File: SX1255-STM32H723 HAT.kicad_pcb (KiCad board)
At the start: 2 copper layers, 77 x 44.2 mm, 36 parts, among them IC1 SX1255, J1 TX_ANT, J2 RX_ANT, J3 STM-L, J4 STM-R, U1 MCP1703Ax-330xxMB, X1 TA0692A, Y1 32MHz

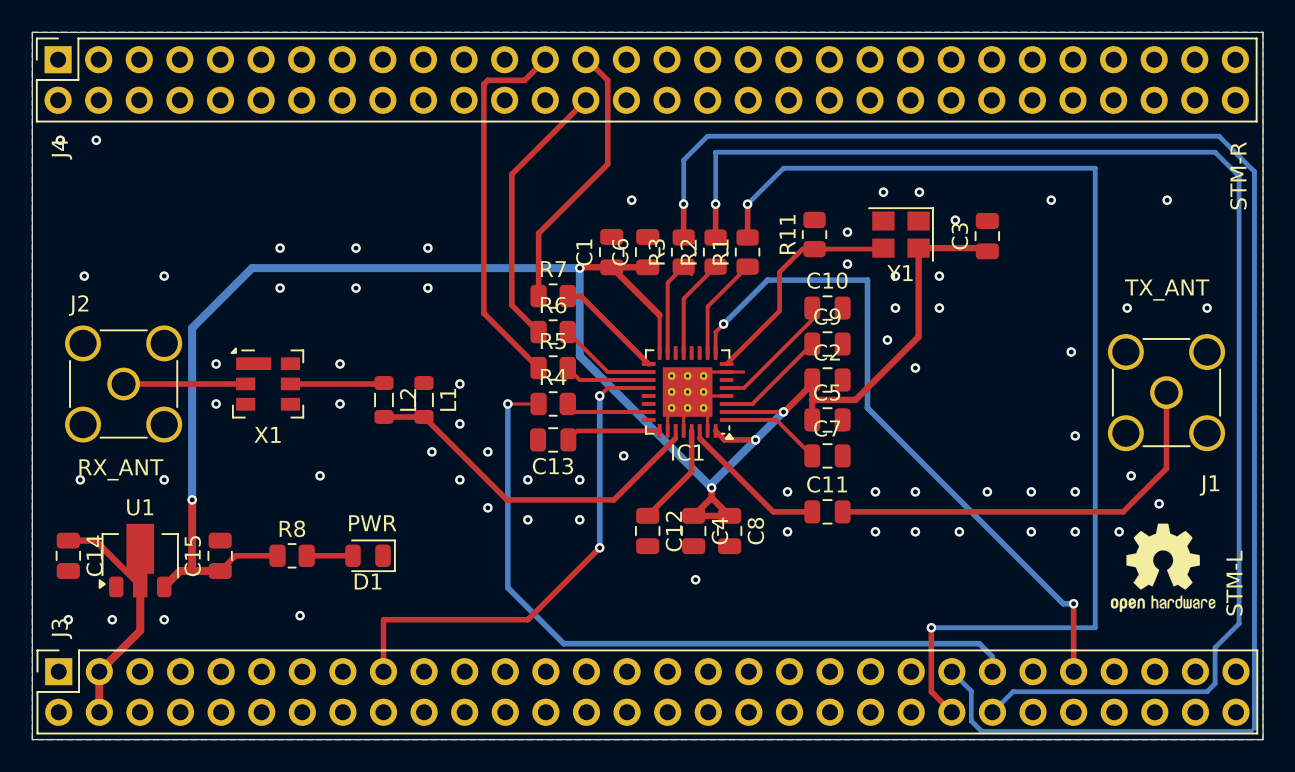
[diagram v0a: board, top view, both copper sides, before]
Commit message: Add files via upload
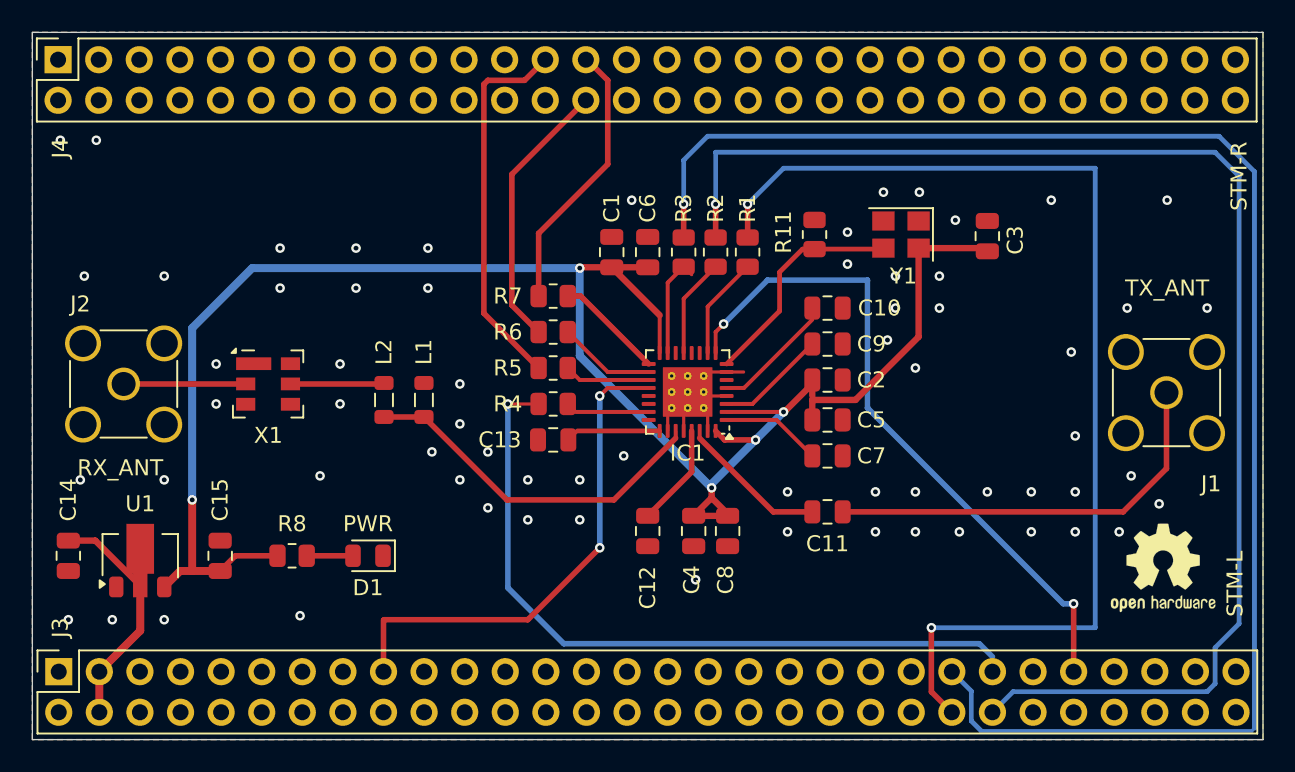
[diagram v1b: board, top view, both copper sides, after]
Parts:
- moved C8 0.12 mm to (147.0, 84.2)
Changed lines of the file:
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@@
 		(tags "resistor")
 		(property "Reference" "R1"
-			(at 0 -1.65 90)
+			(at 2.75 0 90)
 			(layer "F.SilkS")
 			(effects
@@
 		)
 		(property "Value" "100R"
-			(at 0 1.65 90)
+			(at 5.75 0 90)
 			(layer "F.Fab")
 			(effects
@@
 		(tags "capacitor")
 		(property "Reference" "C5"
-			(at 0 -1.68 0)
+			(at 2.75 0 0)
 			(layer "F.SilkS")
 			(effects
@@
 		)
 		(property "Value" "100n"
-			(at 0 1.68 0)
+			(at -3.5 0 0)
 			(layer "F.Fab")
 			(effects
@@
 		(tags "resistor")
 		(property "Reference" "R5"
-			(at 0 -1.65 0)
+			(at -2.8375 0 0)
 			(layer "F.SilkS")
 			(effects
@@
 		)
 		(property "Value" "100R"
-			(at 0 1.65 0)
+			(at 3.6625 0 0)
 			(layer "F.Fab")
 			(effects
@@
 		(tags "capacitor")
 		(property "Reference" "C14"
-			(at 0 -1.68 90)
+			(at -3.5 0 90)
 			(layer "F.SilkS")
 			(effects
@@
 		)
 		(property "Value" "1u"
-			(at 0 1.68 90)
+			(at -3.5 -1.5 90)
 			(layer "F.Fab")
 			(effects
@@
 		(tags "capacitor")
 		(property "Reference" "C11"
-			(at 0 -1.68 0)
+			(at 0 2 0)
 			(layer "F.SilkS")
 			(effects
@@
 		)
 		(property "Value" "33p"
-			(at 0 1.68 0)
+			(at 0 -1.75 0)
 			(layer "F.Fab")
 			(effects
@@
 		(tags "capacitor")
 		(property "Reference" "C2"
-			(at 0 -1.68 0)
+			(at 2.75 0 0)
 			(layer "F.SilkS")
 			(effects
@@
 		)
 		(property "Value" "10n"
-			(at 0 1.68 0)
+			(at -3 0 0)
 			(layer "F.Fab")
 			(effects
@@
 		(tags "capacitor")
 		(property "Reference" "C13"
-			(at 0 -1.68 0)
+			(at 3.3375 0 0)
 			(layer "F.SilkS")
 			(effects
@@
 		)
 		(property "Value" "100n"
-			(at 0 1.68 0)
+			(at -3.6625 0 0)
 			(layer "F.Fab")
 			(effects
@@
 		(tags "resistor")
 		(property "Reference" "R7"
-			(at 0 -1.65 0)
+			(at -2.8375 0 0)
 			(layer "F.SilkS")
 			(effects
@@
 		)
 		(property "Value" "100R"
-			(at 0 1.65 0)
+			(at 3.6625 0 0)
 			(layer "F.Fab")
 			(effects
@@
 		(tags "inductor")
 		(property "Reference" "L1"
-			(at 0 -1.55 90)
+			(at -3 0 90)
 			(layer "F.SilkS")
 			(effects
@@
 		)
 		(property "Value" "82n"
-			(at 0 1.55 90)
+			(at 3.25 0 90)
 			(layer "F.Fab")
 			(effects
@@
 		(tags "capacitor")
 		(property "Reference" "C3"
-			(at 0 -1.68 90)
+			(at -0.25 1.75 90)
 			(layer "F.SilkS")
 			(effects
@@
 		)
 		(property "Value" "10n"
-			(at 0 1.68 90)
+			(at 3.5 0 90)
 			(layer "F.Fab")
 			(effects
@@
 		(tags "capacitor")
 		(property "Reference" "C7"
-			(at 0 -1.68 0)
+			(at 2.75 0 0)
 			(layer "F.SilkS")
 			(effects
@@
 		)
 		(property "Value" "100n"
-			(at 0 1.68 0)
+			(at -3.5 0 0)
 			(layer "F.Fab")
 			(effects
@@
 		(tags "SMD SMT crystal")
 		(property "Reference" "Y1"
-			(at 0 -2.45 0)
+			(at -0.15 -2.6 0)
 			(layer "F.SilkS")
 			(effects
@@
 		)
 		(property "Value" "32MHz"
-			(at 0 2.45 0)
+			(at -0.15 2.65 0)
 			(layer "F.Fab")
 			(effects
@@
 		(tags "LED")
 		(property "Reference" "D1"
-			(at 0 -1.65 0)
+			(at 0 -2 0)
 			(layer "F.SilkS")
 			(effects
@@
 		)
 		(property "Value" "PWR"
-			(at -0.25 2 0)
+			(at 0 2 0)
 			(layer "F.SilkS")
 			(effects
@@
 		(tags "resistor")
 		(property "Reference" "R8"
-			(at 0 -1.65 0)
+			(at 0 -2 0)
 			(layer "F.SilkS")
 			(effects
@@
 		)
 		(property "Value" "100R"
-			(at 0 1.65 0)
+			(at 0 2 0)
 			(layer "F.Fab")
 			(effects
@@
 		(tags "capacitor")
 		(property "Reference" "C4"
-			(at 0 -1.68 90)
+			(at 3.05 0.125 90)
 			(layer "F.SilkS")
 			(effects
@@
 		)
 		(property "Value" "10n"
-			(at 0 1.68 90)
+			(at -2.95 0.125 90)
 			(layer "F.Fab")
 			(effects
@@
 		(tags "resistor")
 		(property "Reference" "R6"
-			(at 0 -1.65 0)
+			(at -2.8375 0 0)
 			(layer "F.SilkS")
 			(effects
@@
 		)
 		(property "Value" "100R"
-			(at 0 1.65 0)
+			(at 3.6625 0 0)
 			(layer "F.Fab")
 			(effects
@@
 		(tags "capacitor")
 		(property "Reference" "C15"
-			(at 0 -1.68 90)
+			(at 3.5 0 90)
 			(layer "F.SilkS")
 			(effects
@@
 		)
 		(property "Value" "1u"
-			(at 0 1.68 90)
+			(at 3.5 1.5 90)
 			(layer "F.Fab")
 			(effects
@@
 		(tags "resistor")
 		(property "Reference" "R2"
-			(at 0 -1.65 90)
+			(at 2.75 0 90)
 			(layer "F.SilkS")
 			(effects
@@
 		)
 		(property "Value" "100R"
-			(at 0 1.65 90)
+			(at 5.75 0 90)
 			(layer "F.Fab")
 			(effects
@@
 		(tags "SOT-89-3")
 		(property "Reference" "U1"
-			(at 3 0 180)
+			(at 3.25 0 180)
 			(layer "F.SilkS")
 			(effects
@@
 		(tags "resistor")
 		(property "Reference" "R4"
-			(at 0 -1.65 0)
+			(at -2.8375 0 0)
 			(layer "F.SilkS")
 			(effects
@@
 		)
 		(property "Value" "100R"
-			(at 0 1.65 0)
+			(at 3.6625 0 0)
 			(layer "F.Fab")
 			(effects
@@
 		(tags "resistor")
 		(property "Reference" "R3"
-			(at 0 -1.65 90)
+			(at 2.75 0 90)
 			(layer "F.SilkS")
 			(effects
@@
 		)
 		(property "Value" "100R"
-			(at 0 1.65 90)
+			(at 5.75 0 90)
 			(layer "F.Fab")
 			(effects
@@
 		(tags "capacitor")
 		(property "Reference" "C6"
-			(at 0 -1.68 90)
+			(at 2.75 0 90)
 			(layer "F.SilkS")
 			(effects
@@
 		)
 		(property "Value" "100n"
-			(at 0 1.68 90)
+			(at 5.75 0 90)
 			(layer "F.Fab")
 			(effects
@@
 		(tags "capacitor")
 		(property "Reference" "C12"
-			(at 0 -1.68 90)
+			(at 3.55 0 90)
 			(layer "F.SilkS")
 			(effects
@@
 		)
 		(property "Value" "27p"
-			(at 0 1.68 90)
+			(at -3.2 0 90)
 			(layer "F.Fab")
 			(effects
@@
 		(tags "capacitor")
 		(property "Reference" "C9"
-			(at 0 -1.68 0)
+			(at 2.75 0 0)
 			(layer "F.SilkS")
 			(effects
@@
 		)
 		(property "Value" "100n"
-			(at 0 1.68 0)
+			(at -3.5 0 0)
 			(layer "F.Fab")
 			(effects
@@
 		(tags "inductor")
 		(property "Reference" "L2"
-			(at 0 -1.55 90)
+			(at -3 0 90)
 			(layer "F.SilkS")
 			(effects
@@
 		)
 		(property "Value" "39n"
-			(at 0 1.55 90)
+			(at 3.25 0 90)
 			(layer "F.Fab")
 			(effects
@@
 		(tags "capacitor")
 		(property "Reference" "C10"
-			(at 0 -1.68 0)
+			(at 3.25 0 0)
 			(layer "F.SilkS")
 			(effects
@@
 		)
 		(property "Value" "100n"
-			(at 0 1.68 0)
+			(at -3.5 0 0)
 			(layer "F.Fab")
 			(effects
@@
 	(footprint "Capacitor_SMD:C_0805_2012Metric"
 		(layer "F.Cu")
-		(at 147.125 84.2 -90)
+		(at 147 84.2 -90)
 		(descr "Capacitor SMD 0805 (2012 Metric), square (rectangular) end terminal, IPC_7351 nominal, (Body size source: IPC-SM-782 page 76, https://www.pcb-3d.com/wordpress/wp-content/uploads/ipc-sm-782a_amendment_1_and_2.pdf, https://docs.google.com/spreadsheets/d/1BsfQQcO9C6DZCsRaXUlFlo91Tg2WpOkGARC1WS5S8t0/edit?usp=sharing), generated with kicad-footprint-generator")
 		(tags "capacitor")
 		(property "Reference" "C8"
-			(at 0 -1.68 90)
+			(at 3.05 0.125 90)
 			(layer "F.SilkS")
 			(effects
@@
 		)
 		(property "Value" "100n"
-			(at 0 1.68 90)
+			(at -3.45 -0.25 90)
 			(layer "F.Fab")
 			(effects
@@
 		(tags "resistor")
 		(property "Reference" "R11"
-			(at 0 -1.65 90)
+			(at 0.15 -1.9375 90)
 			(layer "F.SilkS")
 			(effects
@@
 		)
 		(property "Value" "10K"
-			(at 0 1.65 90)
+			(at 3.4 0.0625 90)
 			(layer "F.Fab")
 			(effects
@@
 		(tags "capacitor")
 		(property "Reference" "C1"
-			(at 0 -1.68 90)
+			(at 2.75 0 90)
 			(layer "F.SilkS")
 			(effects
@@
 		)
 		(property "Value" "10n"
-			(at 0 1.68 90)
+			(at 5.25 0 90)
 			(layer "F.Fab")
 			(effects
